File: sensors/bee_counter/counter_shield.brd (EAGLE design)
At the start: 100 x 80 mm, 33 parts

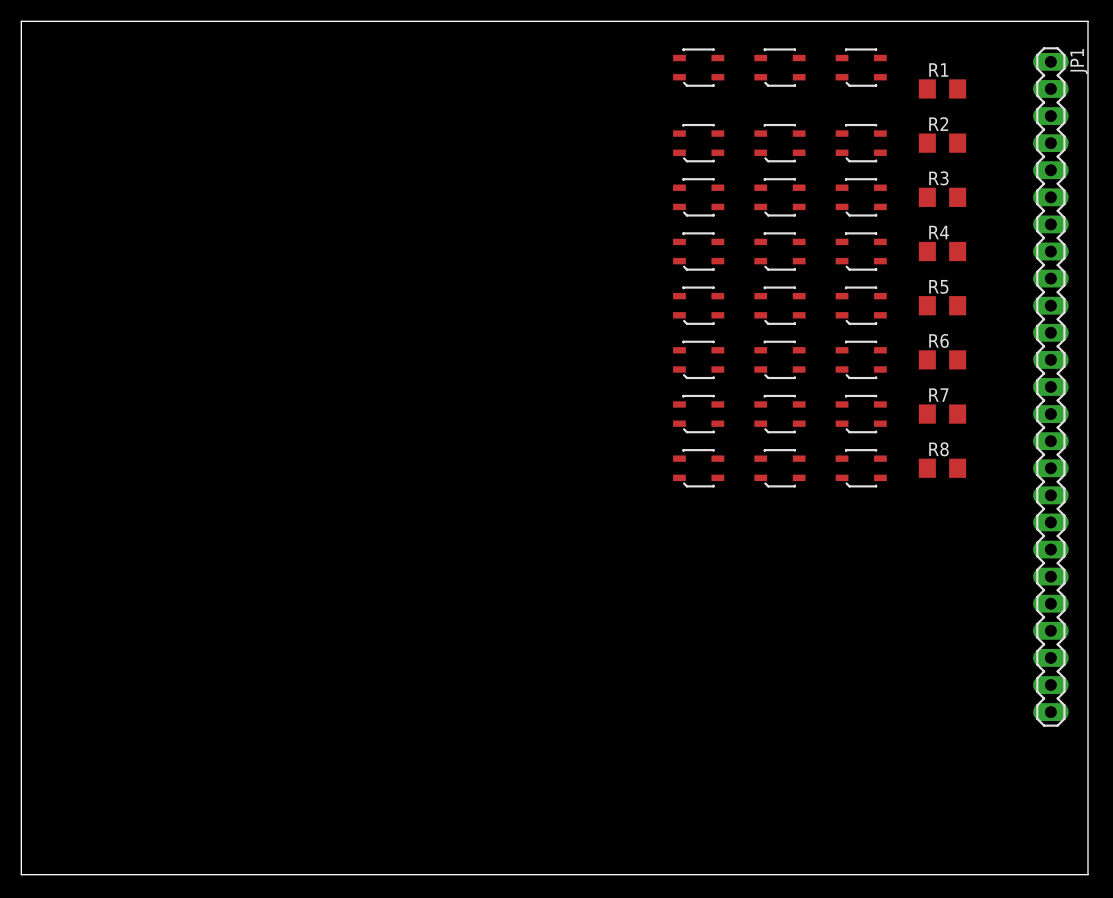
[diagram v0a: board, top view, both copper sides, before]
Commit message: laser stuff
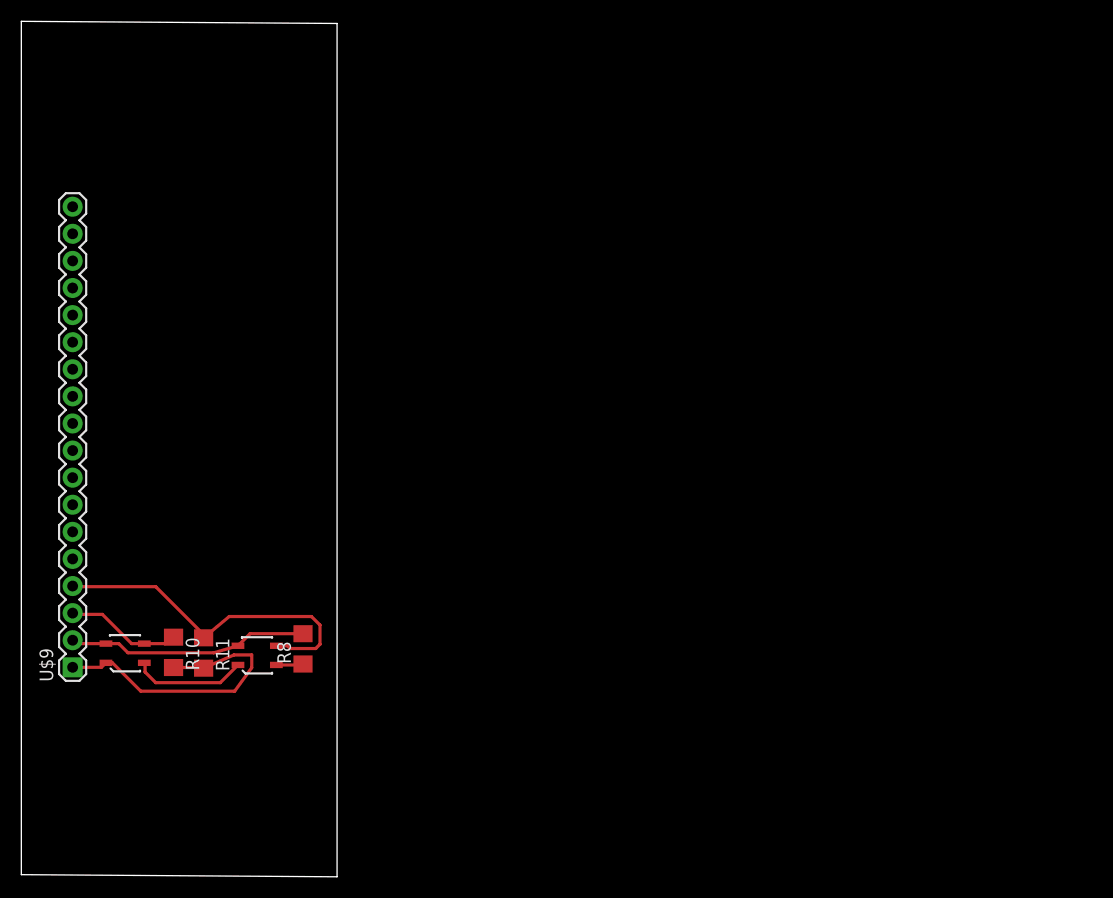
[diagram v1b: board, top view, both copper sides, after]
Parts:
- removed JP1: M25PTH_LONGPADS, SparkFun-Connectors:1X25_LONGPAD
- removed R1, R2, R3, R4, R5, R6, R7: 33, 01_ng:1206
- removed U$1, U$10, U$11, U$12, U$13, U$14, U$15, U$16, U$17, U$18, U$19, U$2, U$20, U$21, U$22, U$23, U$24, U$3, U$4, U$5, U$8: QRE1113, SparkFun-Sensors:QRE1113
- added R10, R11: 10k, 01_ng:1206
- R8: value 33 -> 100
- U$9: value QRE1113 -> M18_; device SparkFun-Sensors:QRE1113 -> SparkFun-Connectors:1X18
- moved U$9 86.9 mm to (4.81, 19.4), turned to 90 degrees
- moved U$7 72.6 mm to (9.73, 20.8)
- moved U$6 63.0 mm to (22.1, 20.6)
- moved R8 62.3 mm to (26.4, 21.2), turned to 90 degrees
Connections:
- removed net N$1: U$17.2, U$9.1
- removed net N$14: U$15.2, U$7.1
- removed net N$15: U$16.2, U$8.1
- removed net N$16: U$16.1, U$24.2
- removed net N$17: R8.1, U$8.2
- removed net N$18: R7.1, U$7.2
- removed net N$19: R6.1, U$6.2
- removed net N$2: U$1.1, U$9.2
- removed net N$20: R5.1, U$5.2
- removed net N$21: R4.1, U$4.2
- removed net N$22: R3.1, U$3.2
- removed net N$23: R2.1, U$2.2
- removed net N$24: R1.1, U$1.2
- removed net N$25: U$17.4
- removed net N$26: U$9.4
- removed net N$27: U$1.4
- removed net N$28: U$18.4
- removed net N$29: U$10.4
- removed net N$3: U$10.1, U$18.2
- removed net N$30: U$2.4
- removed net N$31: U$19.4
- removed net N$32: U$11.4
- removed net N$33: U$3.4
- removed net N$34: U$20.4
- removed net N$35: U$12.4
- removed net N$36: U$4.4
- removed net N$37: U$21.4
- removed net N$38: U$13.4
- removed net N$39: U$5.4
- removed net N$4: U$10.2, U$2.1
- removed net N$40: U$22.4
- removed net N$41: U$14.4
- removed net N$42: U$6.4
- removed net N$43: U$23.4
- removed net N$44: U$15.4
- removed net N$45: U$7.4
- removed net N$46: U$24.4
- removed net N$47: U$16.4
- removed net N$48: U$8.4
- removed net N$5: U$11.2, U$3.1
- removed net N$6: U$11.1, U$19.2
- removed net N$7: U$12.1, U$20.2
- removed net N$8: U$12.2, U$4.1
- removed net N$9: U$13.1, U$21.2
- net GND: now also U$6.4, U$7.4, U$9.2; no longer JP1.2, R1.2, R2.2, R3.2, R4.2, R5.2, R6.2, R7.2
- net N$10: now also R8.1, U$6.2; no longer U$13.2, U$5.1
- net N$11: now also U$7.2; no longer U$14.2
- net N$12: now also R10.1, U$7.3, U$9.3; no longer U$14.1, U$22.2
- net N$13: now also R11.1, U$6.3, U$9.4; no longer U$15.1, U$23.2
- net VCC: now also R10.2, R11.2, U$7.1, U$9.1; no longer JP1.1, U$1.3, U$10.3, U$11.3, U$12.3, U$13.3, U$14.3, U$15.3, U$16.3, U$17.1, U$17.3, U$18.1, U$18.3, U$19.1, U$19.3, U$2.3, U$20.1, U$20.3, U$21.1, U$21.3, U$22.1, U$22.3, U$23.1, U$23.3, U$24.1, U$24.3, U$3.3, U$4.3, U$5.3, U$6.3, U$7.3, U$8.3, U$9.3
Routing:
- net N$13: track 0.00 -> 33.0 mm
- net VCC: track 0.00 -> 28.7 mm
- net GND: track 0.00 -> 22.7 mm
- net N$12: track 0.00 -> 10.8 mm
- net N$11: track 0.00 -> 10.7 mm
- net N$10: track 0.00 -> 2.54 mm
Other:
- board size 100 x 80 mm -> 29.6 x 80.2 mm
